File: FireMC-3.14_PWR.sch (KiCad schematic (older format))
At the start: 71 parts, among them J1 Header_1X2, J2 Header_1X2, Q1 STD86N3LH5, Q2 STD86N3LH5, Q3 STD86N3LH5, Q4 STD86N3LH5, U1 ISL6420B, U2 ISL6420B

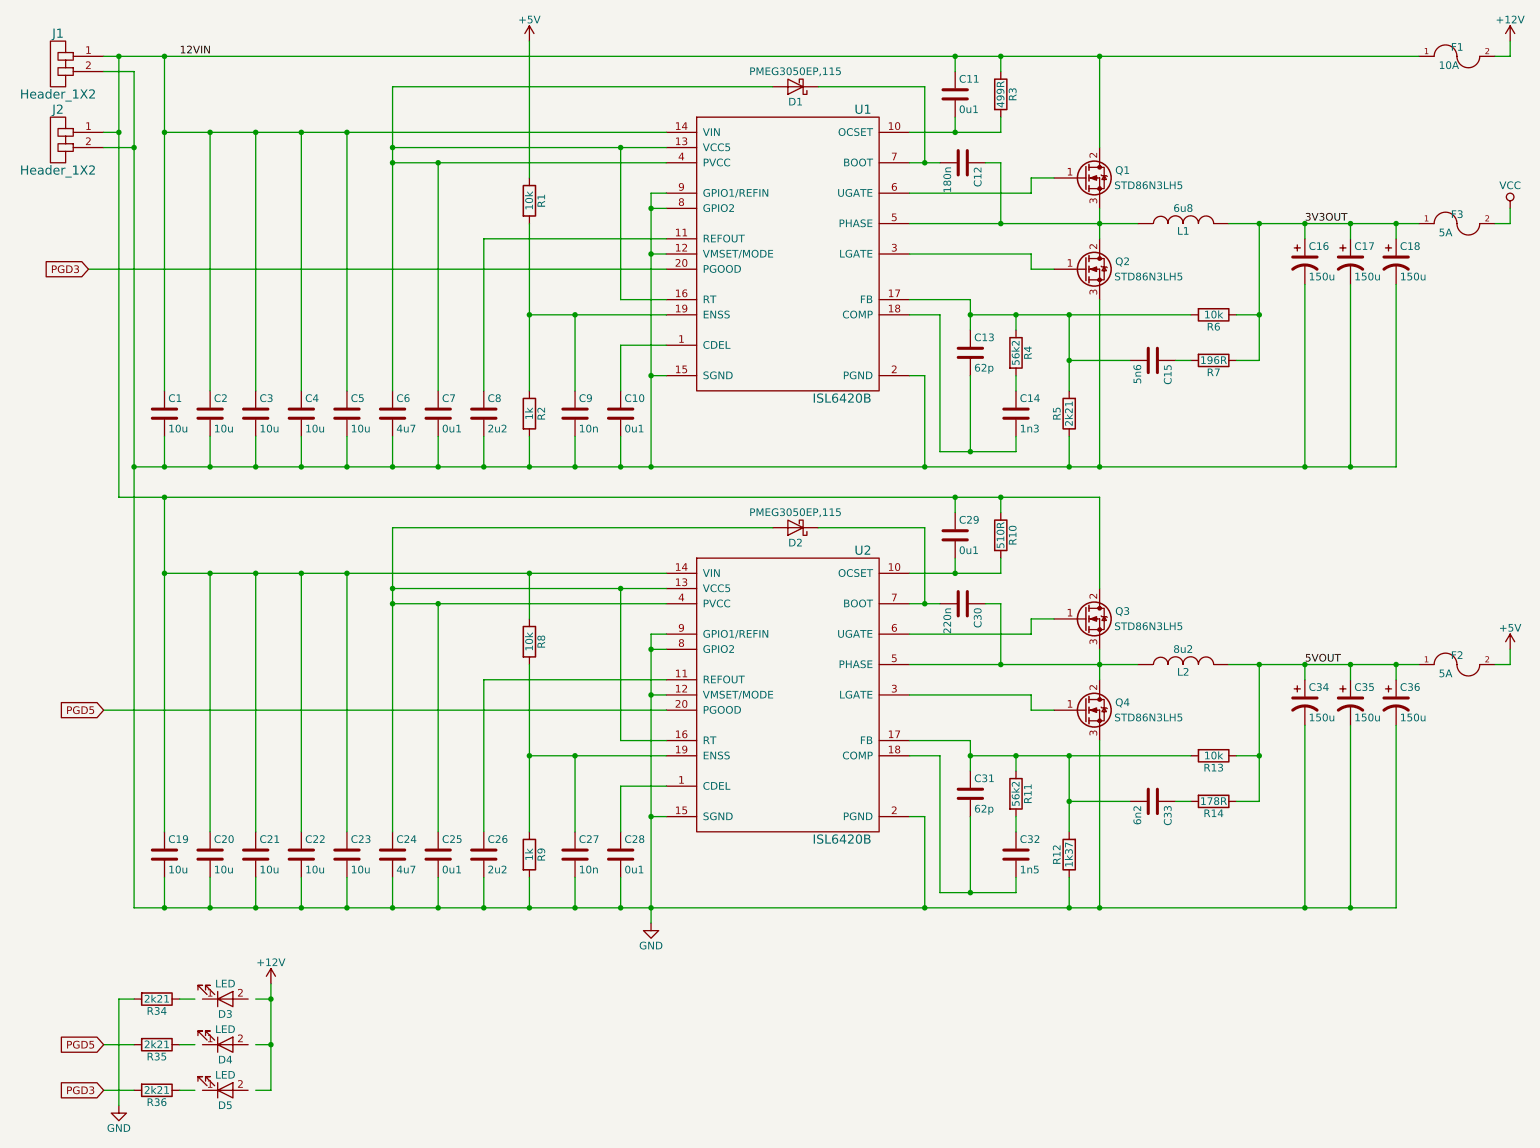
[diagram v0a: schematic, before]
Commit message: Changed Power management
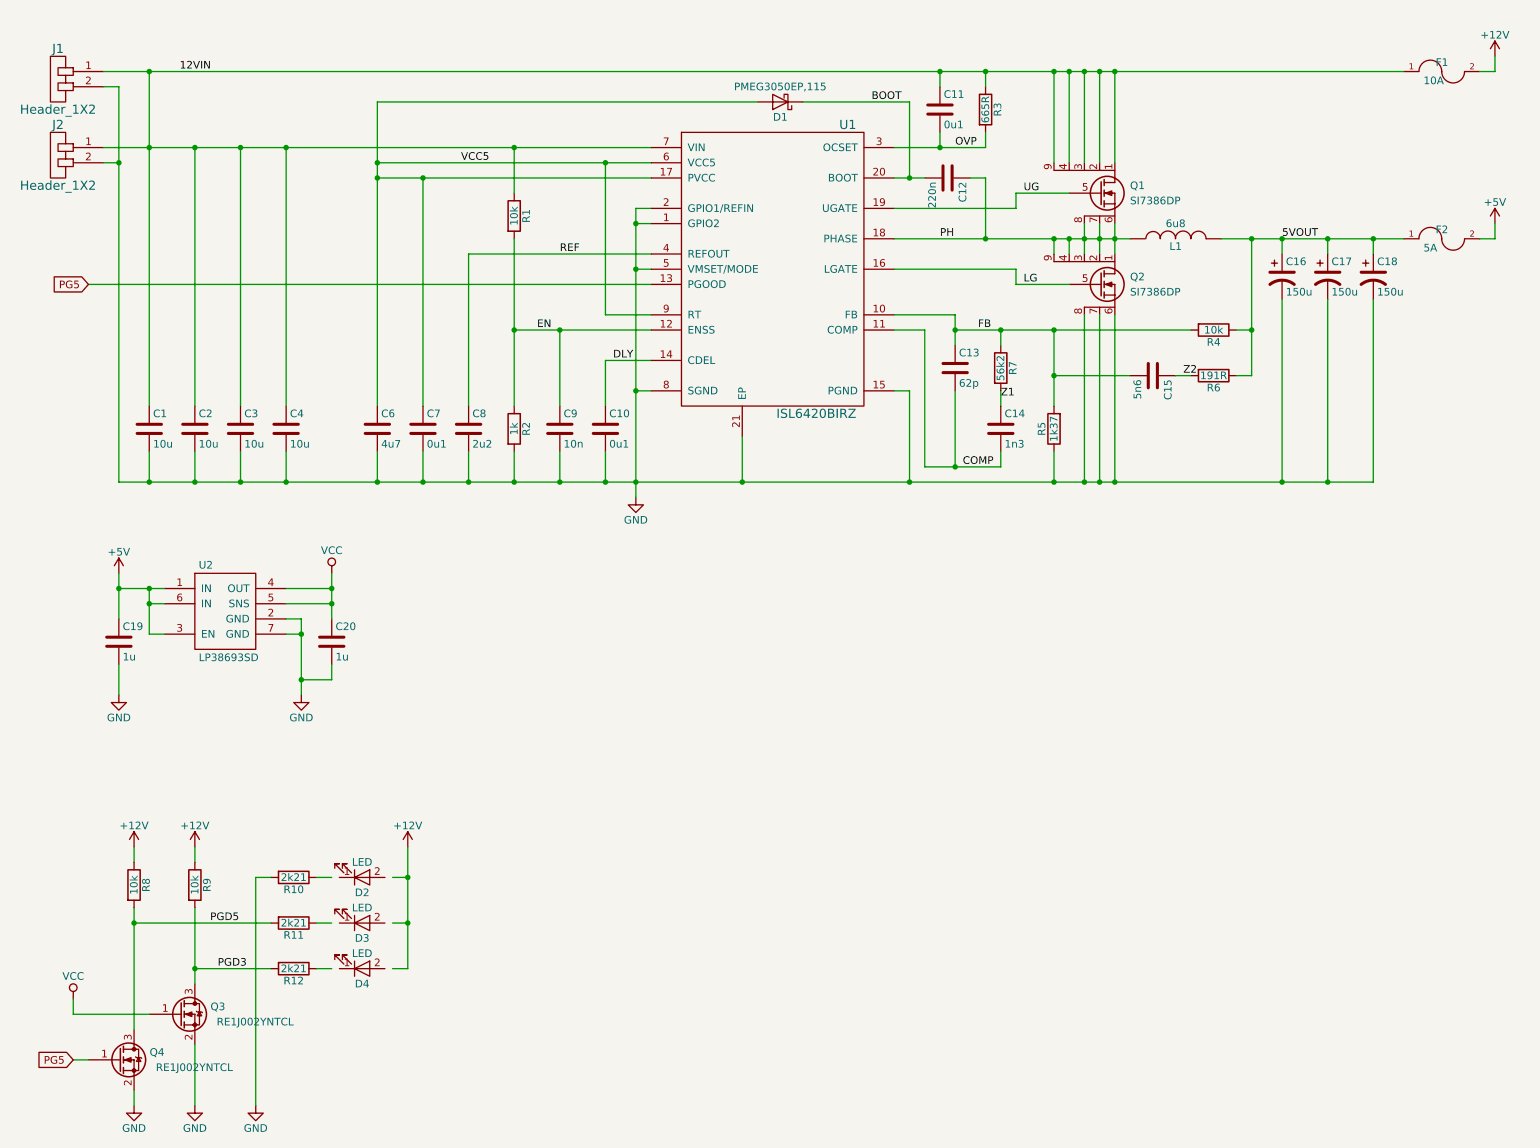
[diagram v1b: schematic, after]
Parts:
- removed C1, C2, C23, C3, C4, C5: 10u, IPC_CAP:CAPC1608X95N, symbol C
- removed C10, C11, C7: 0u1, IPC_CAP:CAPC1608X90N, symbol C
- removed C12: 180n, IPC_CAP:CAPC1608X90N, symbol C
- removed C13: 62p, IPC_CAP:CAPC1608X90N, symbol C
- removed C14: 1n3, IPC_CAP:CAPC1608X90N, symbol C
- removed C15: 5n6, IPC_CAP:CAPC1608X90N, symbol C
- removed C16, C17, C18: 150u, IPC_CAP:CAPAE660X770N, symbol CP1
- removed C6: 4u7, IPC_CAP:CAPC1608X95N, symbol C
- removed C8: 2u2, IPC_CAP:CAPC1608X90N, symbol C
- removed C9: 10n, IPC_CAP:CAPC1608X90N, symbol C
- removed D1: PMEG3050EP,115, IPC_SOD:SOD4725X100N, symbol D_Schottky
- removed F3: 5A, IPC_MFG:MPD_BK-6010, symbol FUSE
- removed L1: 6u8, IPC_IND:INDM1213X620N, symbol INDUCTOR
- removed Q1, Q2, Q3, Q4: STD86N3LH5, IPC_TO:TO228P972X240-3N, symbol Q_NMOS_GDS
- removed R1, R6: 10k, IPC_RES:RESC1608X55N, symbol R
- removed R2: 1k, IPC_RES:RESC1608X55N, symbol R
- removed R3: 499R, IPC_RES:RESC1608X55N, symbol R
- removed R4: 56k2, IPC_RES:RESC1608X55N, symbol R
- removed R5: 2k21, IPC_RES:RESC1608X55N, symbol R
- removed R7: 196R, IPC_RES:RESC1608X55N, symbol R
- removed U1, U2: ISL6420B, IPC_SOP:SOP63P600X155-20N, symbol ISL6420B
- added C19, C20: 1u, IPC_CAP:CAPC1608X90N, symbol C
- added Q1, Q2: SI7386DP, IPC_SON:SON9P127_490X590X112L61X41T376X348N, symbol Q_NMOS_DDDDGSSSD
- added Q3, Q4: RE1J002YNTCL, IPC_SOFL:SOTFL3P50_160X85L45X28N, symbol Q_NMOS_GSD
- added R8, R9: 10k, IPC_RES:RESC1608X55N, symbol R
- added U1: ISL6420BIRZ, IPC_QFN:QFN21P50_400X400X100L55X24T210N, symbol ISL6420BIRZ
- added U2: LP38693SD, IPC_SON:SON7P95_300X300X80L40X35T210X160N, symbol LP38693SD
- C14: renamed from C32; value 1n5 -> 1n3
- C15: renamed from C33; value 6n2 -> 5n6
- L1: renamed from L2; value 8u2 -> 6u8
- R3: renamed from R10; value 510R -> 665R
- R6: renamed from R14; value 178R -> 191R
- renumbered C19 to C1, C28 to C10, C29 to C11, C30 to C12, C31 to C13, C34 to C16, C35 to C17, C36 to C18, C20 to C2, C21 to C3, C22 to C4, C24 to C6, C25 to C7, C26 to C8, C27 to C9, D2 to D1, D3 to D2, D4 to D3, D5 to D4, R8 to R1, R34 to R10, R35 to R11, R36 to R12, R9 to R2, R13 to R4, R12 to R5, R11 to R7
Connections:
- net labels added: BOOT, COMP, DLY, EN, FB, LG, OVP, PG5, PH, REF, UG, VCC5, Z1, Z2
- net labels removed: 3V3OUT
- wire segments 194 -> 136
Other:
- moved on the sheet: C1, C10, C11, C12, C13, C14, C15, C16, C17, C18, C2, C3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

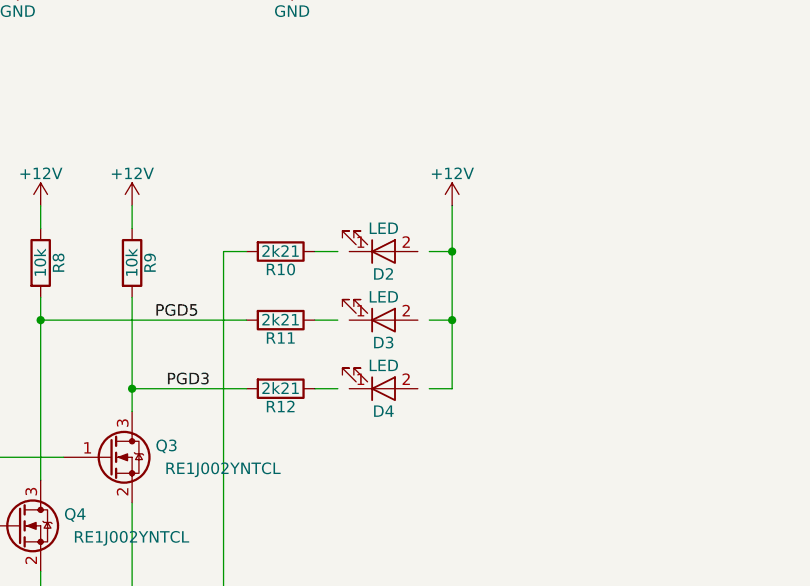
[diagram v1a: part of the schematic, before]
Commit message: KiCAD 4.0.5 Update corrections
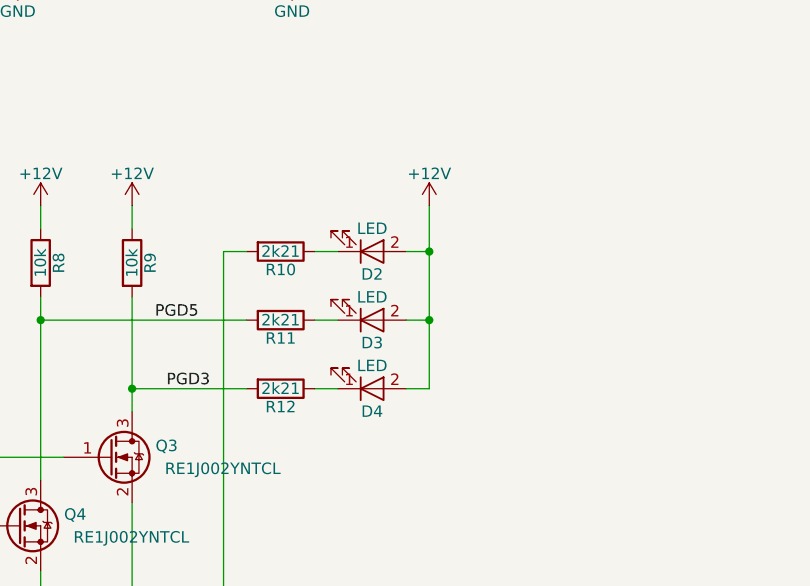
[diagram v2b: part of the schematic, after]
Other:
- moved on the sheet: D2, D3, D4
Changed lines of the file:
@@
 LIBS:microcontrollers
 LIBS:dsp
-LIBS:microchip
+LIBS:Microchip Technologies
 LIBS:analog_switches
 LIBS:motorola
-LIBS:texas
+LIBS:TI
 LIBS:intel
 LIBS:audio
@@
 LIBS:stepstick
 LIBS:Linear Technologies
-LIBS:Microchip Technologies
 LIBS:Maxim Integrated
 LIBS:Intersil
 LIBS:mounting hole
-LIBS:TI
 LIBS:power_transistors
 LIBS:FireMC-3.14-cache
@@
 L LED D2
 U 1 1 57D606BA
-P 2800 6200
-F 0 "D2" H 2800 6300 50  0000 C CNN
-F 1 "LED" H 2800 6100 50  0000 C CNN
-F 2 "IPC_LED:LEDM1608X70N" H 2800 6200 50  0001 C CNN
-F 3 "" H 2800 6200 50  0000 C CNN
-	1    2800 6200
+P 2750 6200
+AR Path="/57D606BA" Ref="D2"  Part="1"
+AR Path="/57C8E291/57D606BA" Ref="D2"  Part="1"
+F 0 "D2" H 2750 6300 50  0000 C CNN
+F 1 "LED" H 2750 6100 50  0000 C CNN
+F 2 "IPC_LED:LEDM1608X70N" H 2750 6200 50  0001 C CNN
+F 3 "" H 2750 6200 50  0000 C CNN
+	1    2750 6200
 	1    0    0    1
 $EndComp
@@
 L LED D3
 U 1 1 57D607A1
-P 2800 6500
-F 0 "D3" H 2800 6600 50  0000 C CNN
-F 1 "LED" H 2800 6400 50  0000 C CNN
-F 2 "IPC_LED:LEDM1608X70N" H 2800 6500 50  0001 C CNN
-F 3 "" H 2800 6500 50  0000 C CNN
-	1    2800 6500
+P 2750 6500
+AR Path="/57D607A1" Ref="D3"  Part="1"
+AR Path="/57C8E291/57D607A1" Ref="D3"  Part="1"
+F 0 "D3" H 2750 6600 50  0000 C CNN
+F 1 "LED" H 2750 6400 50  0000 C CNN
+F 2 "IPC_LED:LEDM1608X70N" H 2750 6500 50  0001 C CNN
+F 3 "" H 2750 6500 50  0000 C CNN
+	1    2750 6500
 	1    0    0    1
 $EndComp
@@
 L LED D4
 U 1 1 57D60886
-P 2800 6800
-F 0 "D4" H 2800 6900 50  0000 C CNN
-F 1 "LED" H 2800 6700 50  0000 C CNN
-F 2 "IPC_LED:LEDM1608X70N" H 2800 6800 50  0001 C CNN
-F 3 "" H 2800 6800 50  0000 C CNN
-	1    2800 6800
+P 2750 6800
+AR Path="/57D60886" Ref="D4"  Part="1"
+AR Path="/57C8E291/57D60886" Ref="D4"  Part="1"
+F 0 "D4" H 2750 6900 50  0000 C CNN
+F 1 "LED" H 2750 6700 50  0000 C CNN
+F 2 "IPC_LED:LEDM1608X70N" H 2750 6800 50  0001 C CNN
+F 3 "" H 2750 6800 50  0000 C CNN
+	1    2750 6800
 	1    0    0    1
 $EndComp
@@
 	2500 6200 2600 6200
 Wire Wire Line
-	3100 6500 3000 6500
-Connection ~ 3100 6200
-Wire Wire Line
-	3100 6800 3000 6800
-Connection ~ 3100 6500
+	3000 6500 2900 6500
+Connection ~ 3000 6200
+Wire Wire Line
+	3000 6800 2900 6800
+Connection ~ 3000 6500
 Wire Wire Line
 	4700 2300 1000 2300
 Wire Wire Line
-	3100 6000 3100 6800
+	3000 6000 3000 6800
 Text Label 1600 900  0    50   ~ 0
 12VIN
@@
 L +12V #PWR05
 U 1 1 58960B20
-P 3100 6000
-F 0 "#PWR05" H 3100 5850 50  0001 C CNN
-F 1 "+12V" H 3100 6140 50  0000 C CNN
-F 2 "" H 3100 6000 50  0000 C CNN
-F 3 "" H 3100 6000 50  0000 C CNN
-	1    3100 6000
+P 3000 6000
+F 0 "#PWR05" H 3000 5850 50  0001 C CNN
+F 1 "+12V" H 3000 6140 50  0000 C CNN
+F 2 "" H 3000 6000 50  0000 C CNN
+F 3 "" H 3000 6000 50  0000 C CNN
+	1    3000 6000
 	1    0    0    -1
 $EndComp
@@
 	2100 7700 2100 6200
 Wire Wire Line
-	3000 6200 3100 6200
+	2900 6200 3000 6200
 Wire Wire Line
 	1200 4300 1500 4300
